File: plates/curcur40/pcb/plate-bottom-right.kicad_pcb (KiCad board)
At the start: 2 copper layers, 125.6 x 88.3 mm, 0 parts

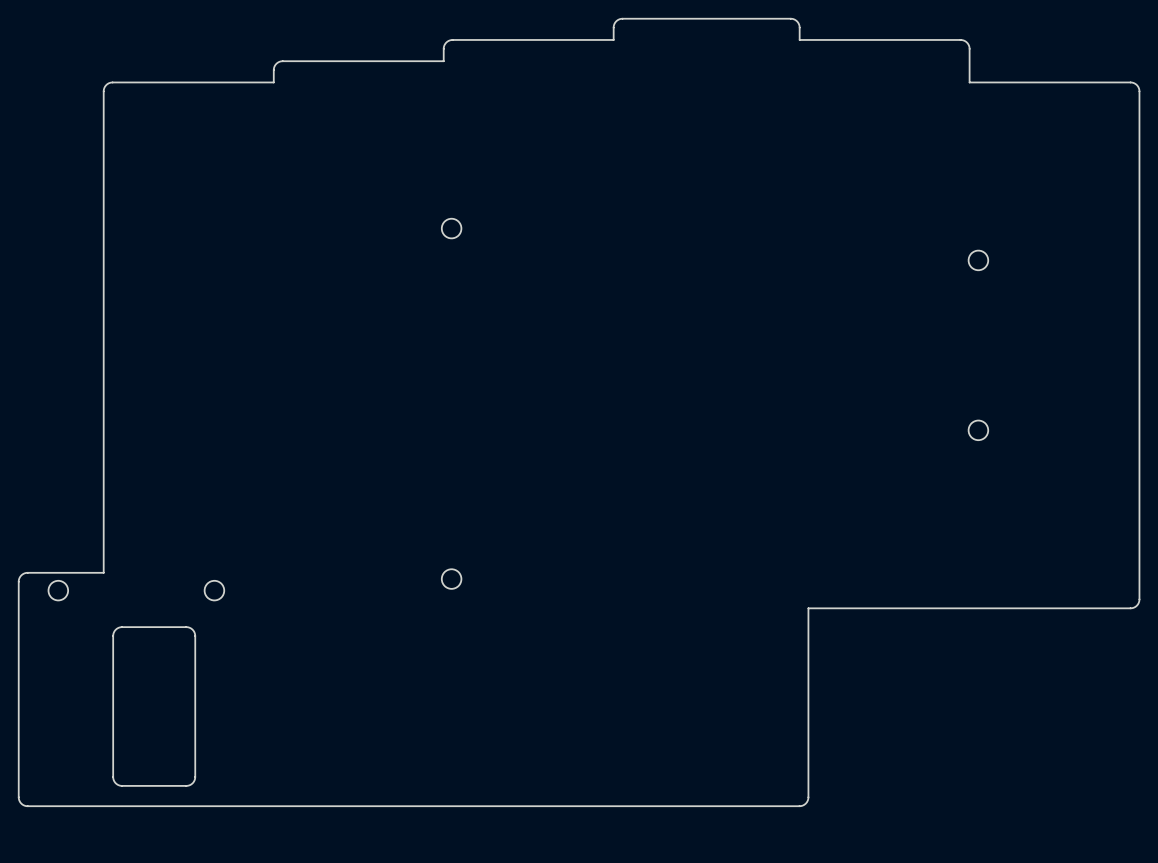
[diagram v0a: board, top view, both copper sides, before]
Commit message: fix all
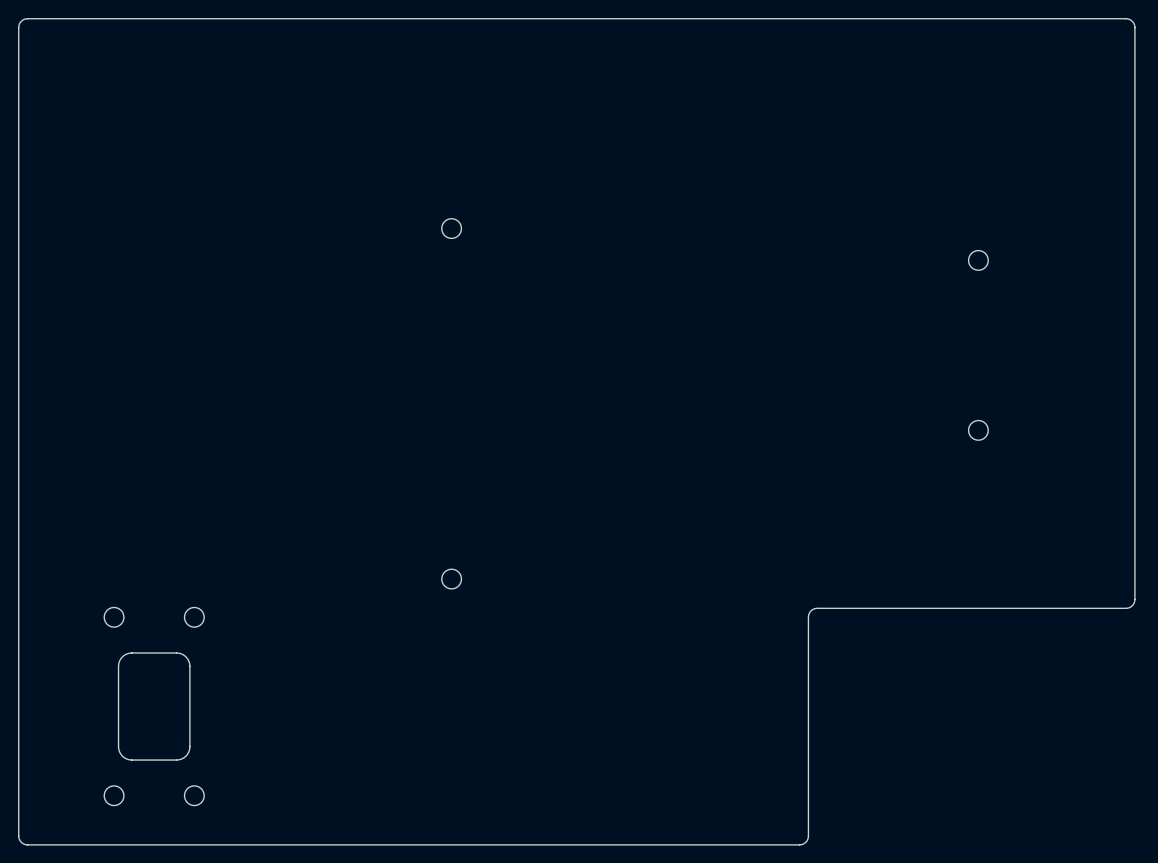
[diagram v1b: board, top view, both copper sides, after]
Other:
- board size 125.6 x 88.3 mm -> 125.1 x 92.6 mm
- rule pad_to_mask_clearance: 0.2 -> 0
